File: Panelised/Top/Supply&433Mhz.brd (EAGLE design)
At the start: 65 x 56.5 mm, 17 parts, among them K1 61004021821, P1 DF11-06-2DSA, Q1 BS170

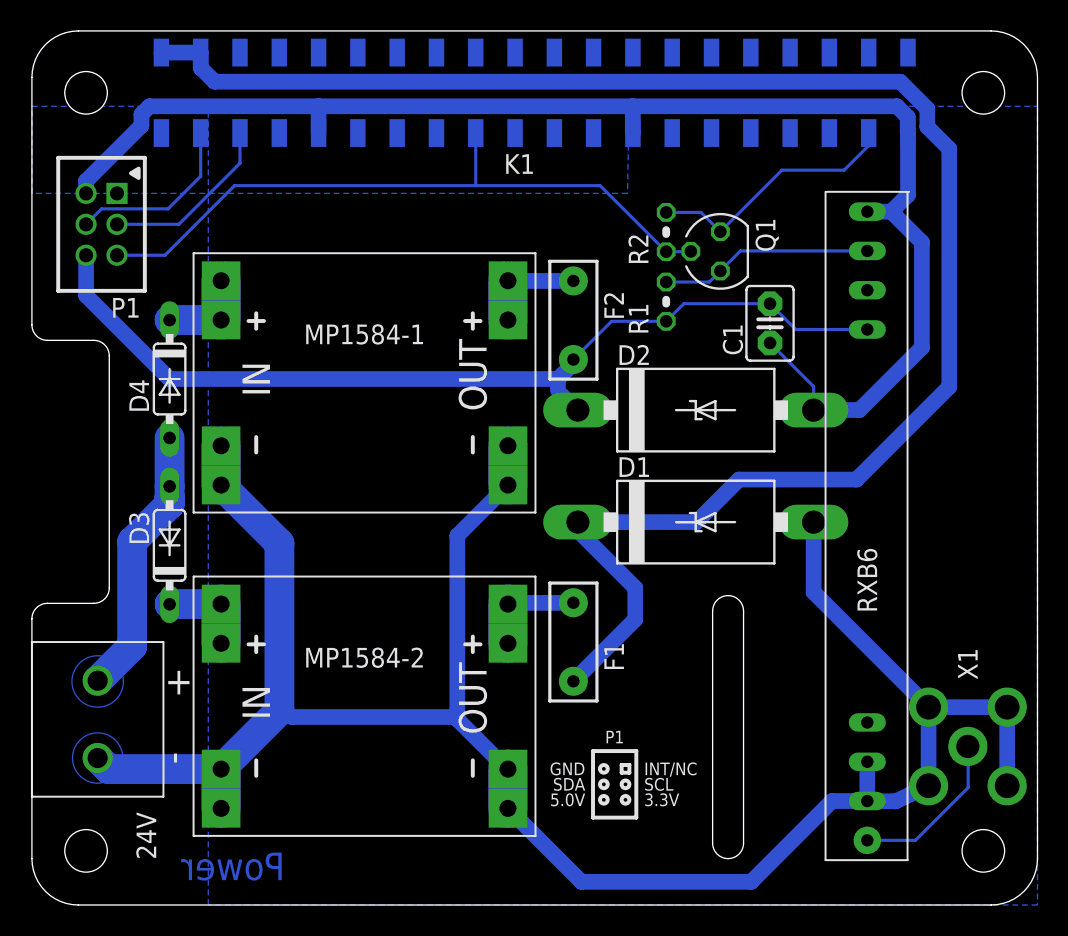
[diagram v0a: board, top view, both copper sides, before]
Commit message: Remove Schottky - Diodes, since already on DC/DC buck converter.
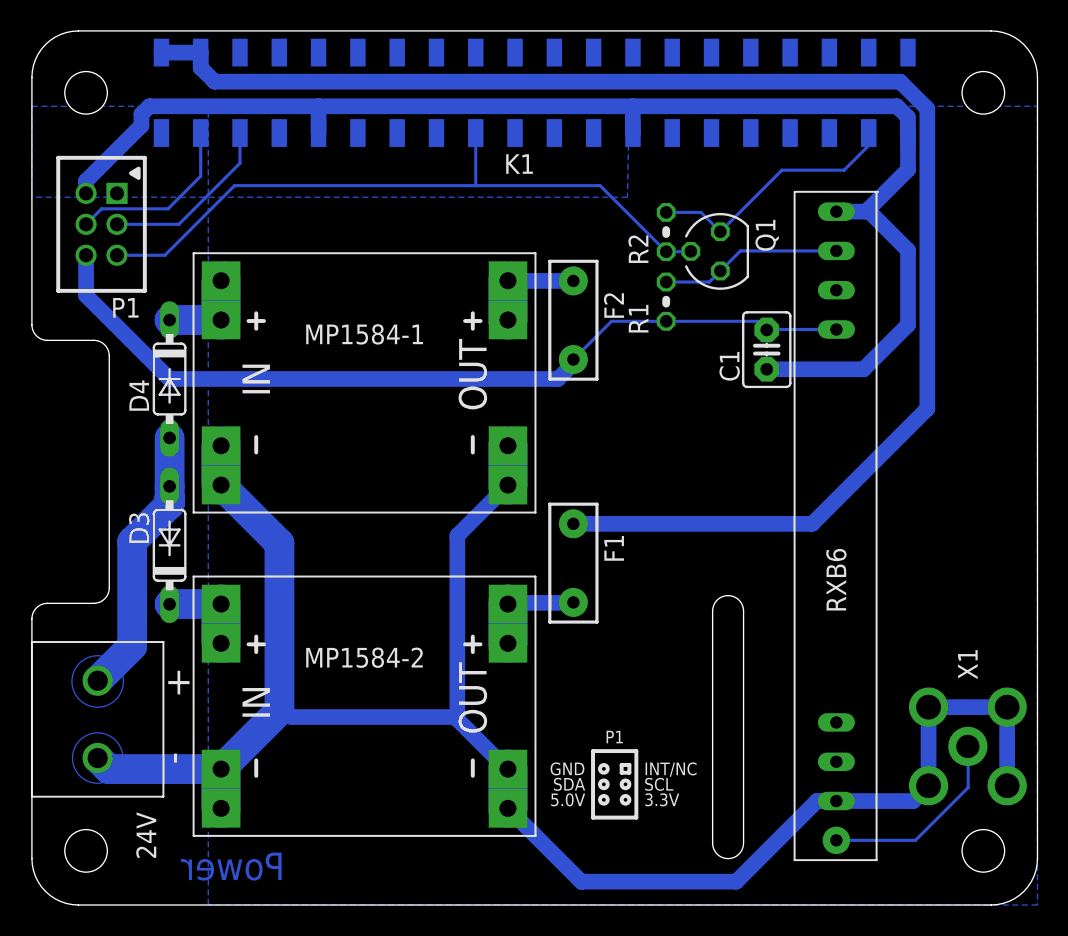
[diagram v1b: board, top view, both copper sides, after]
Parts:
- removed D1, D2: 1N5908, diode:C4111-15
- moved F1 5.10 mm to (35.0, 22.1), turned to 270 degrees
- moved RXB6 2.00 mm to (52.0, 24.5)
- moved C1 1.71 mm to (47.5, 35.9)
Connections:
- net GND: no longer D1.A, D2.A
- net N$2: no longer D2.C
- net N$5: no longer D1.C
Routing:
- net GND: track 229.3 -> 208.0 mm
- net N$5: track 111.3 -> 96.9 mm
- net N$2: track 60.8 -> 55.3 mm
- net N$8: track 10.6 -> 12.6 mm
- net N$3: track 13.8 -> 11.8 mm

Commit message: Revert "Remove Schottky - Diodes, since already on DC/DC buck converter."
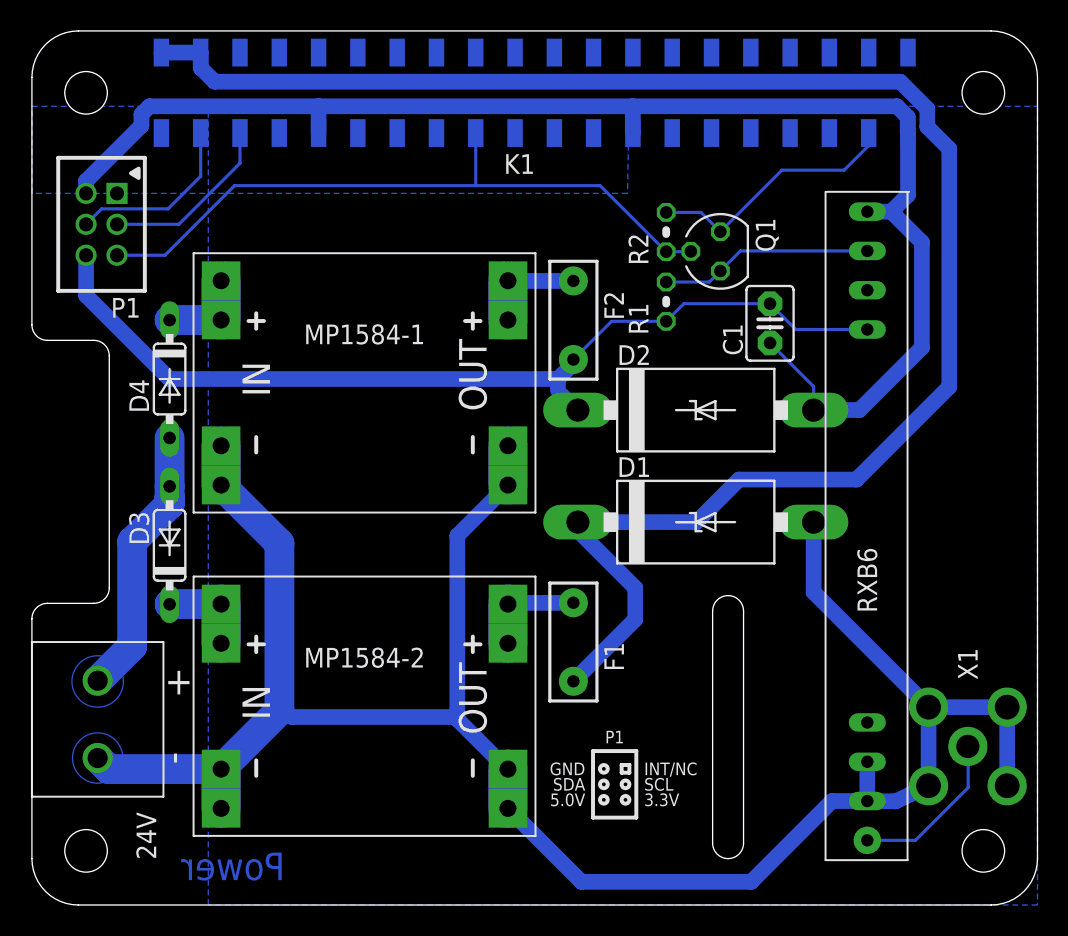
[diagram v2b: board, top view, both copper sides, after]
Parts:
- added D1, D2: 1N5908, diode:C4111-15
- moved F1 5.10 mm to (35.0, 17.0), turned to 90 degrees
- moved RXB6 2.00 mm to (54.0, 24.5)
- moved C1 1.71 mm to (47.7, 37.6)
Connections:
- net GND: now also D1.A, D2.A
- net N$2: now also D2.C
- net N$5: now also D1.C
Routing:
- net GND: track 208.0 -> 229.3 mm
- net N$5: track 96.9 -> 111.3 mm
- net N$2: track 55.3 -> 60.8 mm
- net N$8: track 12.6 -> 10.6 mm
- net N$3: track 11.8 -> 13.8 mm
